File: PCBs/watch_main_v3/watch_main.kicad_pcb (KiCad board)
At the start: 8 copper layers, 37 x 40.5 mm, 121 parts, among them IC1001 S26HS512TGABHI000, IC1101 NVT4858HKZ, IC1301 IIS2MDCTR, IC1302 OPT3004DNPR, IC1801 M24256X-FCU6T_VF, IC201 ADP5360ACBZ-2-R7, IC401 BGA725L6E6327FTSA1, J1101 105162-0001, J1701 10-Pin Pogo Connector, J501 AXG130144, J601 AXG110144A, J701 AXG120144, Q201 DMP2104LP-7, SW1501 EVP-AEJB2A, U101 Watch_Outline_V2, U1102 NCP45525IMNTWG-H, U1301 LSM6DSO16IS, U1401 RT4730WSC, U1601 GPS_&_BT_Antenna_Keepout, U401 TESEO-LIV3FL, Y801 16MHz, Y802 32.768kHz

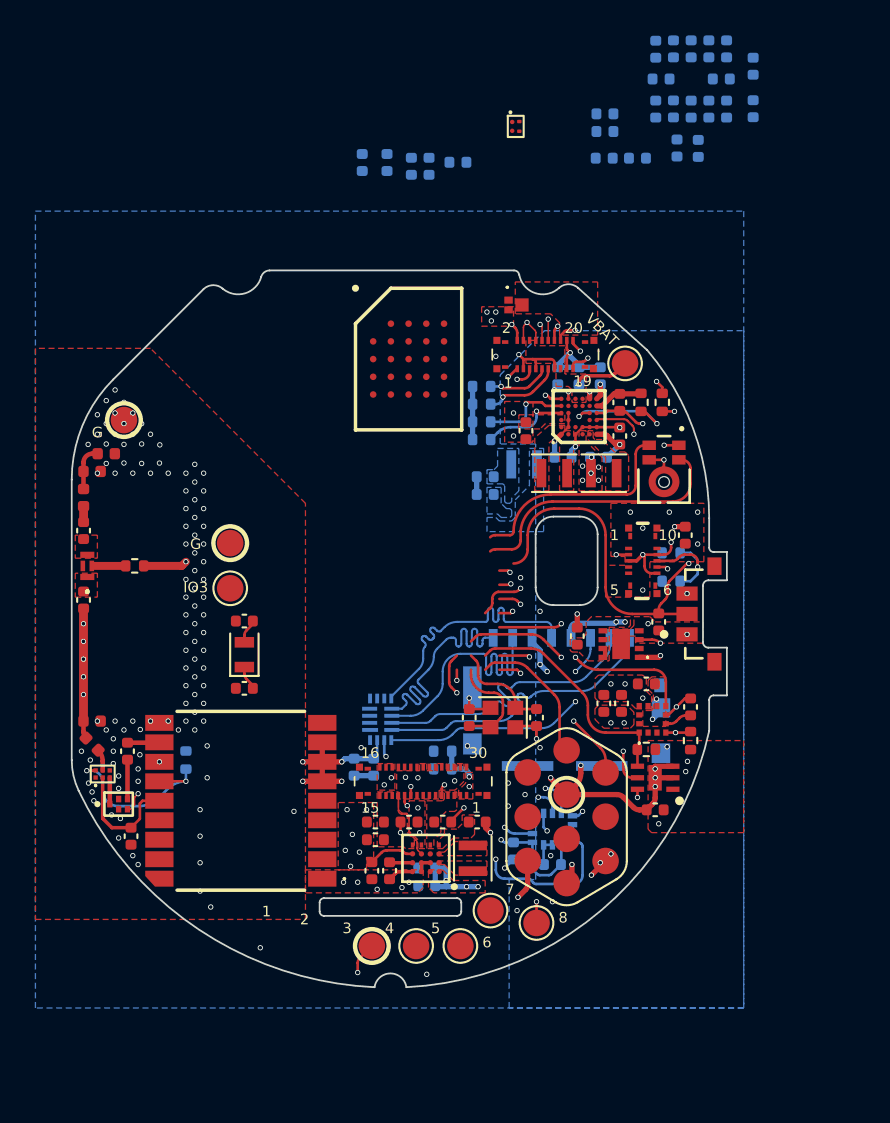
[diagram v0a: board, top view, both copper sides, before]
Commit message: watch_main_v3 updates
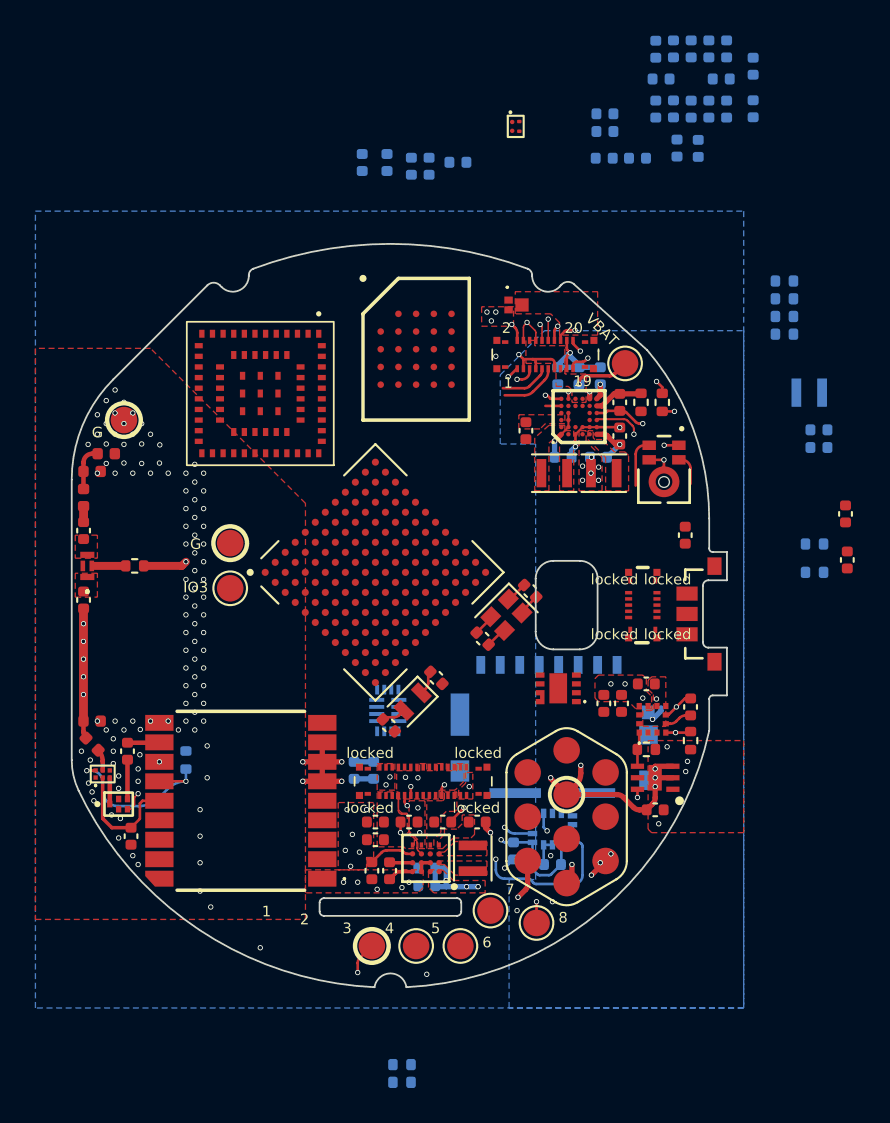
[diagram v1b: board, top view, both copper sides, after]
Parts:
- added REF**: BGA-144_12x12_10.0x10.0mm, watch_footprints:BGA-144_12x12_10.0x10.0mm, F.Cu at (149.2, 95.4)
- added REF**: LBEE5PK2AE-564, watch_footprints:LBEE5PK2AE-564, F.Cu at (142.7, 85.3)
- U101: footprint watch_footprints:Watch Outline V2 -> watch_footprints:Watch Outline V3
- moved C906 19.0 mm to (174.2, 88.3)
- moved C922 19.0 mm to (174.2, 87.3)
- moved R801 18.1 mm to (172.3, 82.0)
- moved R802 18.1 mm to (172.3, 81.0)
- moved R805 18.1 mm to (172.3, 79.0)
- moved R806 18.1 mm to (172.3, 80.0)
- moved R809 17.8 mm to (150.7, 124.2)
- moved R810 17.8 mm to (150.7, 123.2)
- moved C1101 16.6 mm to (175.8, 92.1)
- moved L901 16.6 mm to (173.7, 85.2)
- moved C1501 11.2 mm to (175.8, 94.7)
- moved C804 10.9 mm to (152.6, 101.4), turned to 135 degrees
- moved C803 10.1 mm to (150.0, 104.0), turned to 135 degrees
- moved Y802 9.86 mm to (151.3, 102.7), turned to -135 degrees
- moved R807 8.12 mm to (174.0, 95.4)
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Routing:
- net /STM32/BTN: track 35.1 -> 0.00 mm, vias 3 -> 0
- net /STM32/IMU_INT1: track 30.2 -> 8.45 mm, vias 2 -> 1
- net /SPI1.SCK: track 21.2 -> 0.00 mm, vias 2 -> 0
- net /SPI1.MISO: track 18.8 -> 0.00 mm, vias 2 -> 0
- net /SPI1.CS: track 19.8 -> 1.07 mm
- net /STM32/SWD.RST: track 18.4 -> 1.20 mm, vias 3 -> 1
- net /Micro SD/DAT2: track 16.6 -> 0.00 mm
- net /Micro SD/DAT3: track 16.5 -> 0.00 mm
- net /Micro SD/DAT0: track 16.3 -> 0.00 mm
- net /Micro SD/CLK: track 16.2 -> 0.00 mm
- net /STM32/IMU_INT2: track 17.6 -> 1.69 mm, vias 2 -> 1
- net /Micro SD/DAT1: track 15.9 -> 0.00 mm
- net /STM32/ALS_INT: track 15.4 -> 0.00 mm, vias 2 -> 0
- net /Micro SD/CMD: track 15.1 -> 0.00 mm, vias 2 -> 0
- net /STM32/TOUCH_RST: track 13.9 -> 0.00 mm, vias 1 -> 0
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- removed copper zone on B.Cu, net +1V8
- removed copper zone on F.Cu, net /Micro SD/+3V3_SD
- removed copper zone on B.Cu, net /STM32 Power/VDD11
- removed copper zone on B.Cu, net /STM32 Power/VLXSMPS
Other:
- board size 37 x 40.5 mm -> 37 x 42 mm
- board text added: "locked"
- board text removed: "10"
- board text removed: "15"
- board text removed: "16"
- board text removed: "30"
